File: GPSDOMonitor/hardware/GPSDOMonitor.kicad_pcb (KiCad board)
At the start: 2 copper layers, 150 x 60 mm, 34 parts, among them J1 F31S-1A7L1-11050, Q1 MMBT3904LT1G, U1 TPS563231DRLR, U2 MCP16301T-I_CHY, U3 PIC18LF2550-ISO, U4 SN74HC595BRWNR, U5 SN74HC595BRWNR, X1 ABM8W-20.0000MHZ-4-K1Z-T3

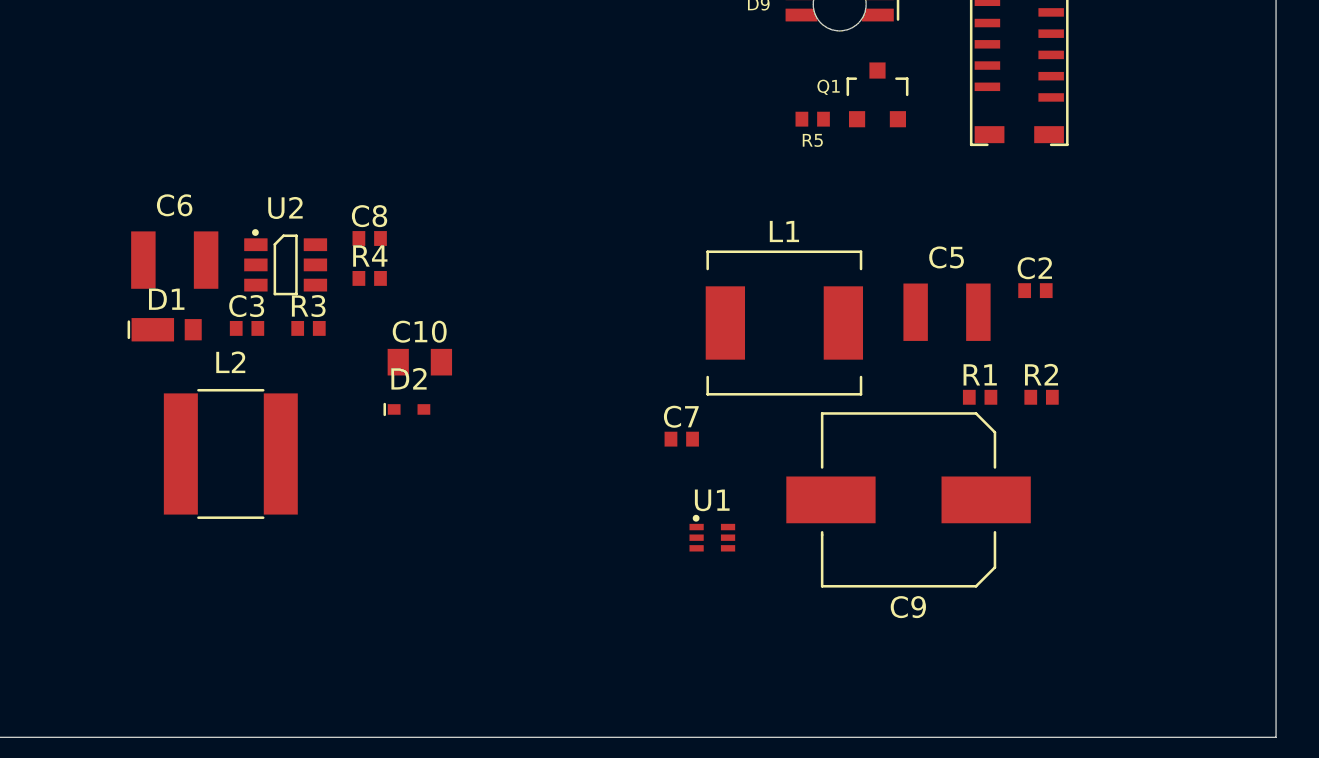
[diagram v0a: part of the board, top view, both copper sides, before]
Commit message: Route power supplies
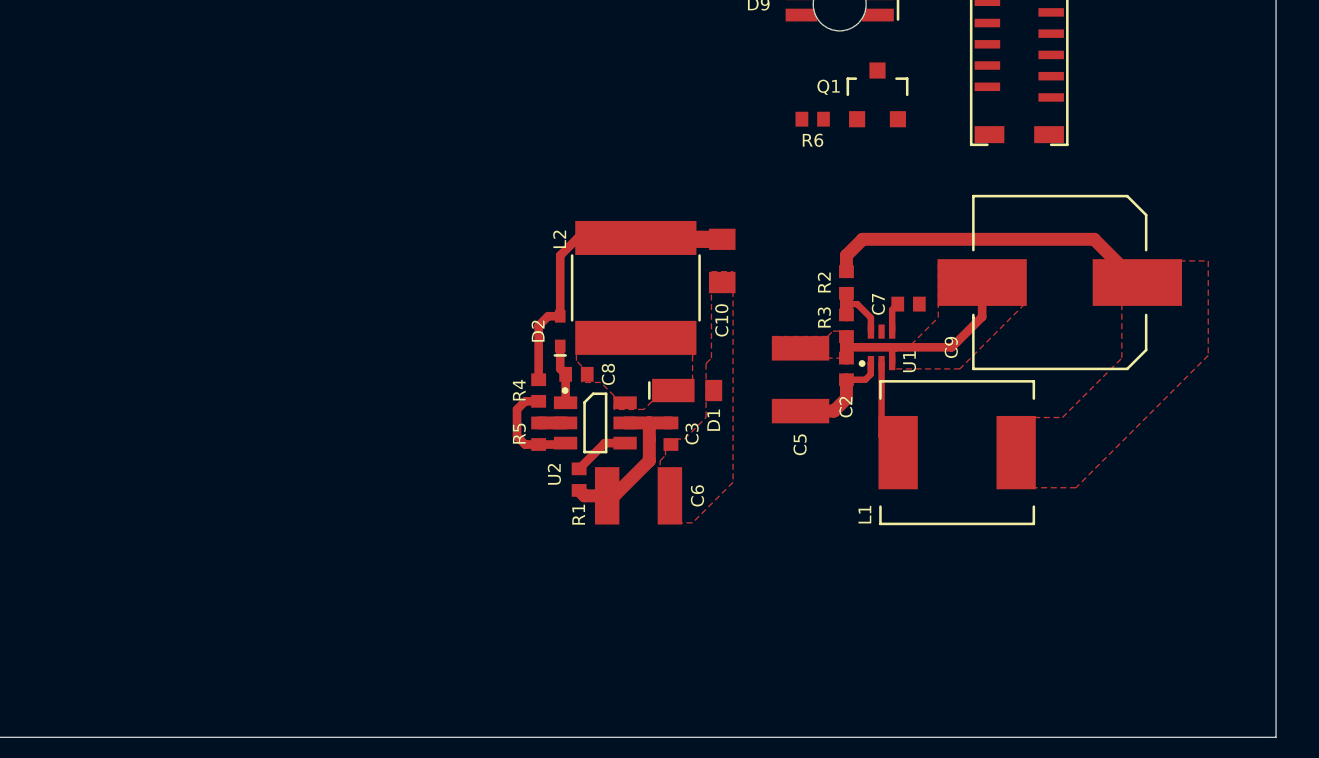
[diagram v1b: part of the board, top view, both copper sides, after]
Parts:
- removed the R3 at (148.1, 78.9)
- added R1: CRG0402ZR, Resistor:R_0402_1005Metric, F.Cu at (160.8, 86.0)
- added R4: CRGCQ0402F33K, Resistor:R_0402_1005Metric, F.Cu at (158.9, 81.8)
- moved D1 24.6 mm to (165.9, 81.8)
- moved C6 24.5 mm to (163.6, 86.7)
- moved L2 20.6 mm to (163.4, 77.0), turned to 90 degrees
- moved C3 20.5 mm to (165.1, 83.8), turned to 270 degrees
- moved U2 16.4 mm to (161.5, 83.3)
- moved C10 15.0 mm to (167.5, 75.7), turned to 270 degrees
- moved C9 12.5 mm to (183.4, 76.7)
- moved C7 12.4 mm to (176.3, 77.7)
- moved U1 12.0 mm to (175.0, 79.8), turned to 90 degrees
- moved C8 11.6 mm to (160.7, 81.0)
- moved R5 10.8 mm to (158.9, 83.8), turned to 90 degrees
- moved L1 10.2 mm to (178.6, 84.7)
- moved R3 9.77 mm to (173.4, 78.7), turned to 270 degrees
- moved C2 9.62 mm to (173.4, 80.8), turned to 90 degrees
- moved R2 8.29 mm to (173.4, 76.7), turned to 270 degrees
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- renumbered R1 to R2, R2 to R3, R4 to R5, R5 to R6
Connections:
- U2 pad 4: +12V -> Net-(R1-Pad2)
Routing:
- net +5V5: track 0.00 -> 15.6 mm
- net +3V3: track 0.00 -> 14.6 mm
- net +12V: track 0.00 -> 13.1 mm
- net GND: track 0.00 -> 11.7 mm
- net Net-(R4-Pad2): track 0.00 -> 4.91 mm
- net Net-(C7-Pad2): track 0.00 -> 4.54 mm
- net Net-(R2-Pad2): track 0.00 -> 3.08 mm
- net Net-(C8-Pad1): track 0.00 -> 2.77 mm
- net Net-(R1-Pad2): track 0.00 -> 2.66 mm
- net Net-(C7-Pad1): track 0.00 -> 1.40 mm
- added copper zone on F.Cu, net +5V5
- added copper zone on F.Cu, net GND
- added copper zone on F.Cu, net Net-(C8-Pad2)
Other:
- net class Default: clearance 0.2 -> 0.1; trace_width 0.25 -> 0.1524; via_dia 0.8 -> 0.508; via_drill 0.4 -> 0.3048
- rule pad_to_mask_clearance: 0 -> 0.05
- rule trace_clearance: 0.2 -> 0.1
- rule trace_min: 0.2 -> 0.1524
- rule via_min_drill: 0.3 -> 0.1524
- rule via_min_size: 0.4 -> 0.1524
